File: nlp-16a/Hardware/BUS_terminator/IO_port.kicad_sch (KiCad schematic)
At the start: 18 parts, among them U1 CD74HC00, U10 CD74HC245, U11 CD74HC00, U12 CD74HC00, U2 CD74HC00, U3 CD74HC00, U4 CD74HC00, U5 CD74HC00, U6 CD74HC00, U7 CD74HC00, U8 CD74HC00, U9 CD74HC245

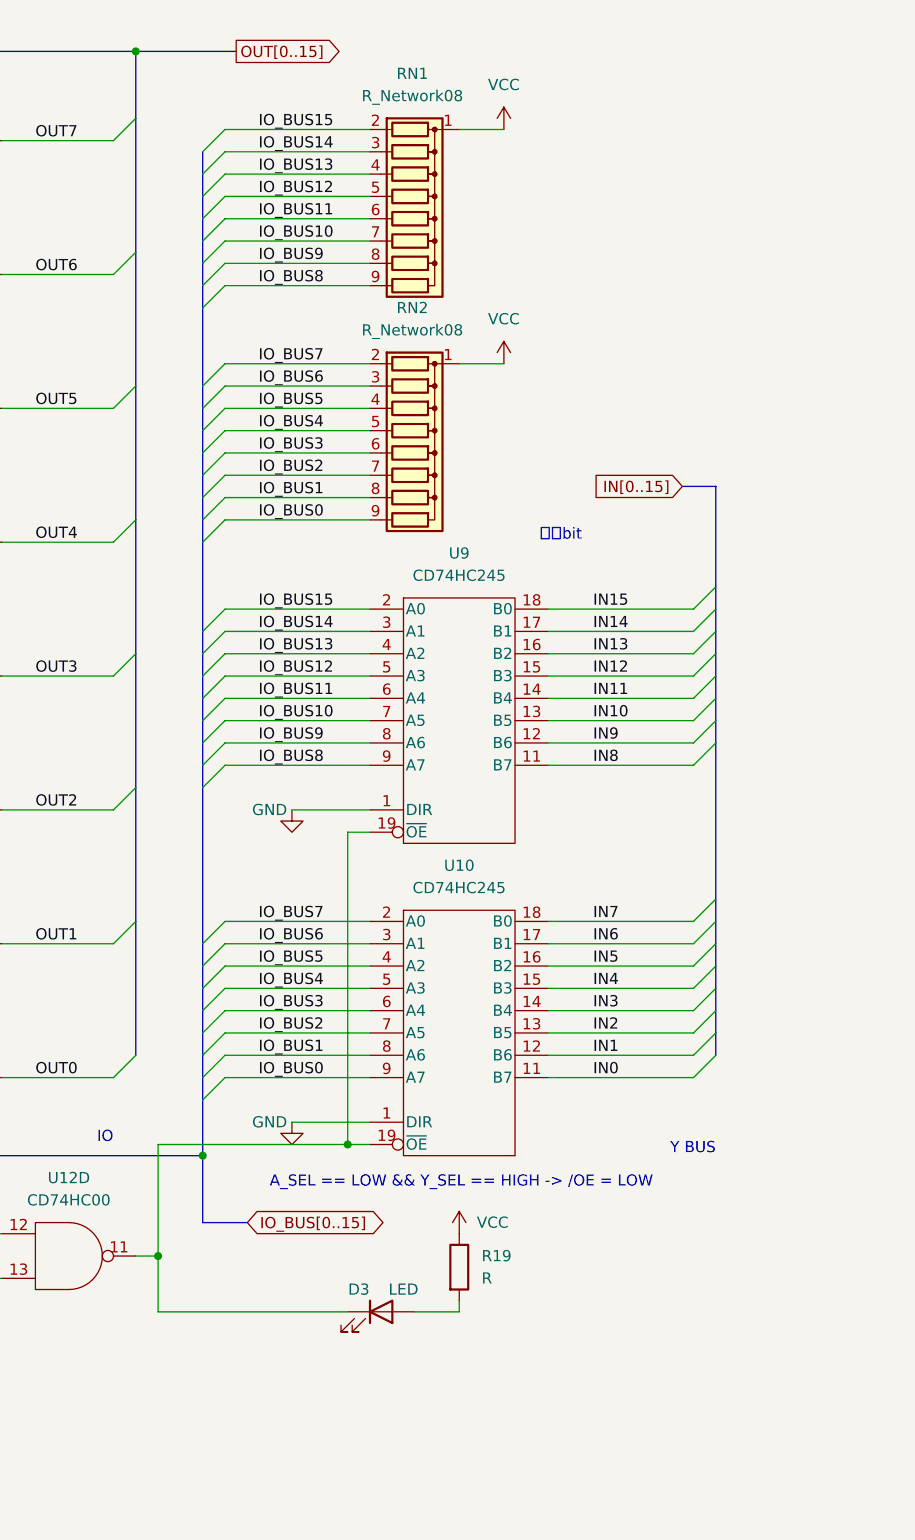
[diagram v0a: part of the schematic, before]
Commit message: アキュムレータ更新
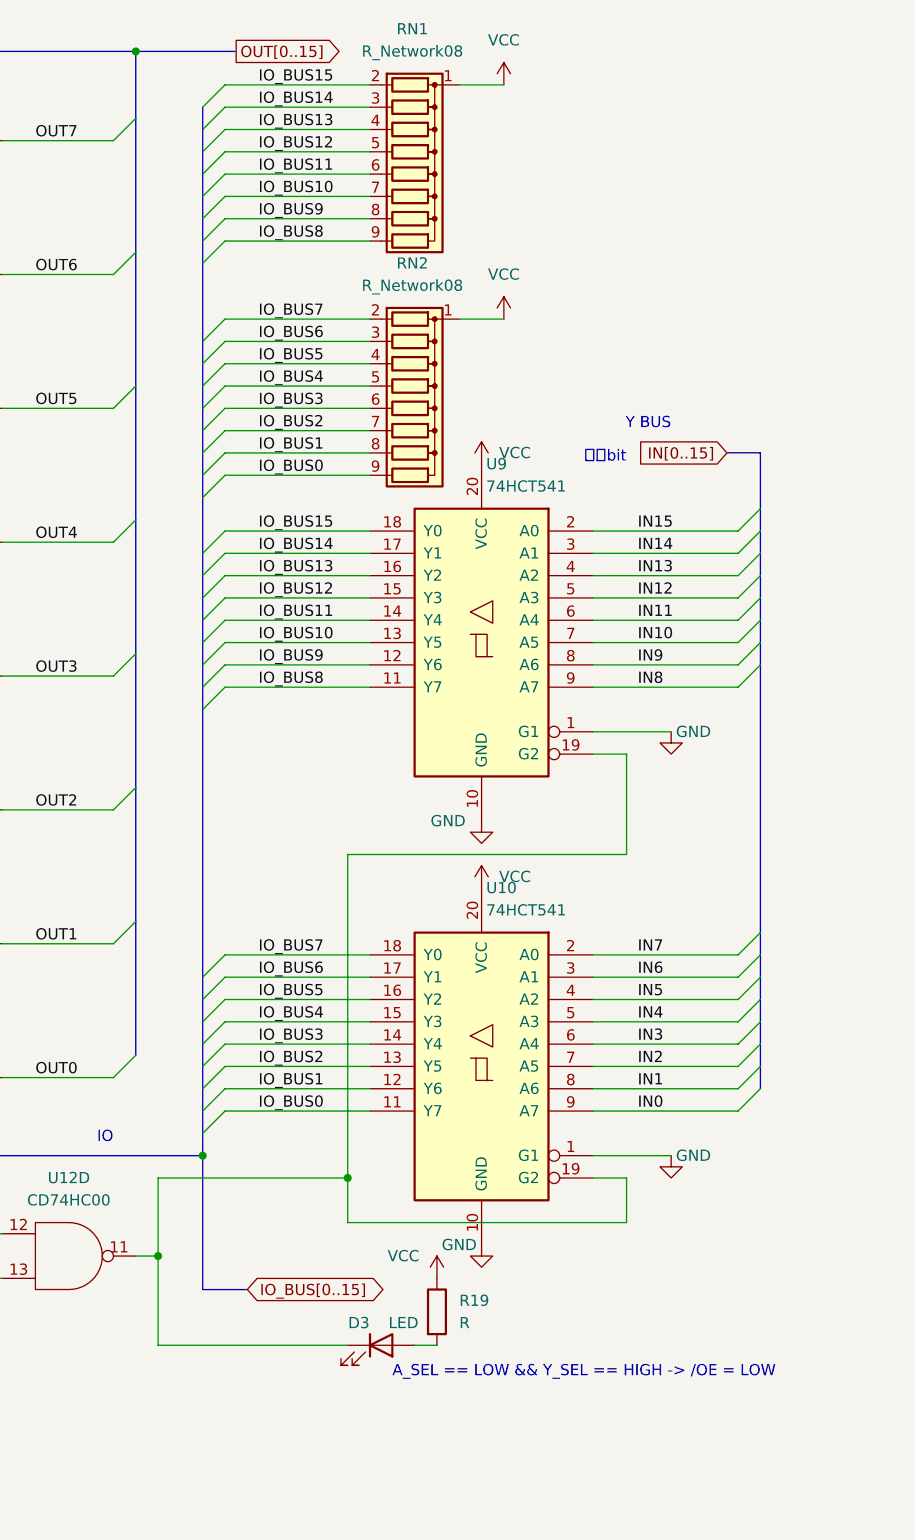
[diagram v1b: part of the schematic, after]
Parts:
- removed U10, U9: CD74HC245, Package_DIP:DIP-20_W7.62mm, symbol CD74HCXX:CD74HC245
- added U10, U9: 74HCT541, Package_DIP:DIP-20_W7.62mm, symbol 74xx:74HCT541
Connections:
- net GND: now also U10.1 (G1), U10.10 (GND), U9.1 (G1), U9.10 (GND)
- net IN0: now also U10.9 (A7)
- net IN1: now also U10.8 (A6)
- net IN10: now also U9.7 (A5)
- net IN11: now also U9.6 (A4)
- net IN12: now also U9.5 (A3)
- net IN13: now also U9.4 (A2)
- net IN14: now also U9.3 (A1)
- net IN15: now also U9.2 (A0)
- net IN2: now also U10.7 (A5)
- net IN3: now also U10.6 (A4)
- net IN4: now also U10.5 (A3)
- net IN5: now also U10.4 (A2)
- net IN6: now also U10.3 (A1)
- net IN7: now also U10.2 (A0)
- net IN8: now also U9.9 (A7)
- net IN9: now also U9.8 (A6)
- net IO_BUS0: now also U10.11 (Y7)
- net IO_BUS1: now also U10.12 (Y6)
- net IO_BUS10: now also U9.13 (Y5)
- net IO_BUS11: now also U9.14 (Y4)
- net IO_BUS12: now also U9.15 (Y3)
- net IO_BUS13: now also U9.16 (Y2)
- net IO_BUS14: now also U9.17 (Y1)
- net IO_BUS15: now also U9.18 (Y0)
- net IO_BUS2: now also U10.13 (Y5)
- net IO_BUS3: now also U10.14 (Y4)
- net IO_BUS4: now also U10.15 (Y3)
- net IO_BUS5: now also U10.16 (Y2)
- net IO_BUS6: now also U10.17 (Y1)
- net IO_BUS7: now also U10.18 (Y0)
- net IO_BUS8: now also U9.11 (Y7)
- net IO_BUS9: now also U9.12 (Y6)
- net VCC: now also U10.20 (VCC), U9.20 (VCC)
- net at D3.1 (K), U12.11: now also U10.19 (G2), U9.19 (G2)
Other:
- moved on the sheet: D3, R19, RN1, RN2
